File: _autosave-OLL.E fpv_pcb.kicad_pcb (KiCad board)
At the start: 6 copper layers, 47.6 x 41.5 mm, 141 parts, among them J1 Micro_SD_Card, J10 Conn_01x05_Pin, J2 RC, J8 reciver, J9 TYPE-C-31-M-12, M1 M1 front left, M2 M2 front right, M3 M3 rear right, M4 m4 rear left, Q1 2N7002, Q2 SUD45P03-09, SW1 SW_SPST, SW2 SW_SPST, U1 MP2315GJ, U10 AON7410, U11 UCC27511ADBV, U12 AON7410, U13 BMP280, U14 STM32H753VITx, U15 USBLC6-2SC6, U3 MP2315GJ, U4 ICM-42688-P, U5 UCC27511ADBV, U6 ul_AON7410, U7 UCC27511ADBV, U8 AON7410, U9 UCC27511ADBV, Y2 8HMz

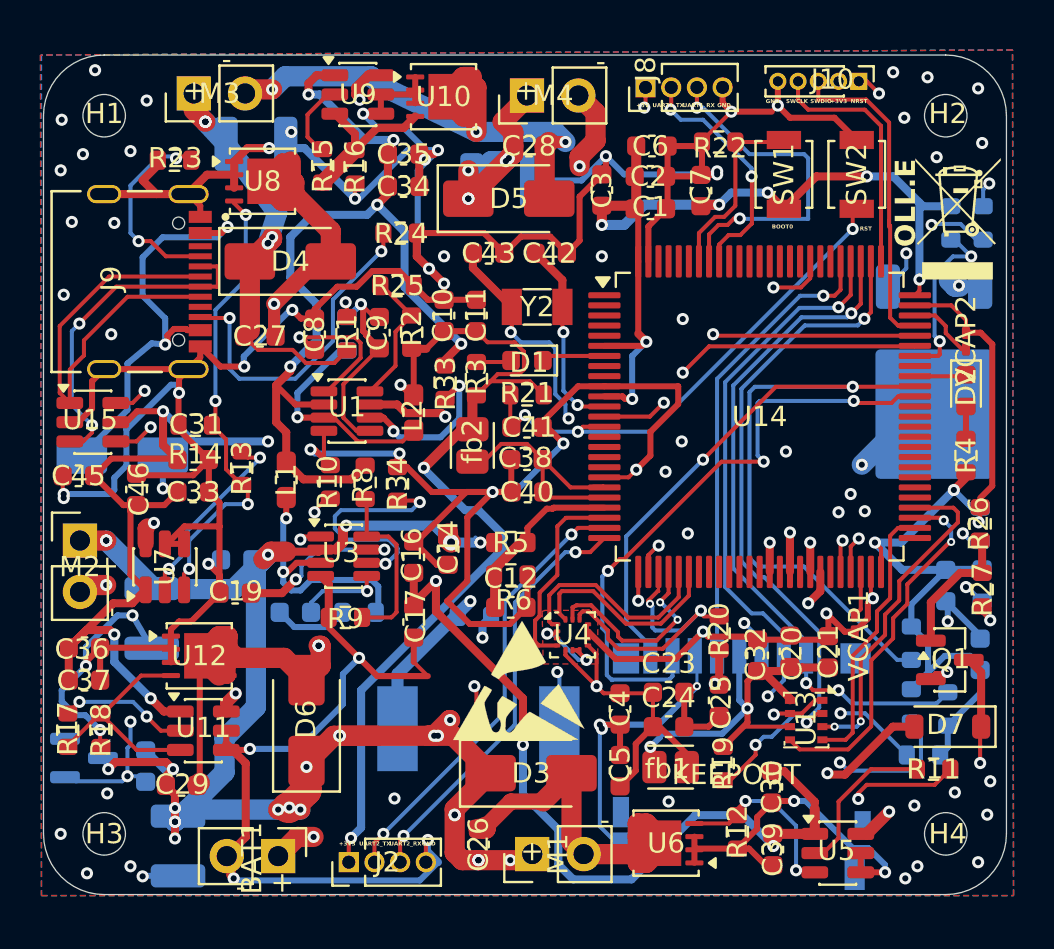
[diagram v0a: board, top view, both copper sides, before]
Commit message: update
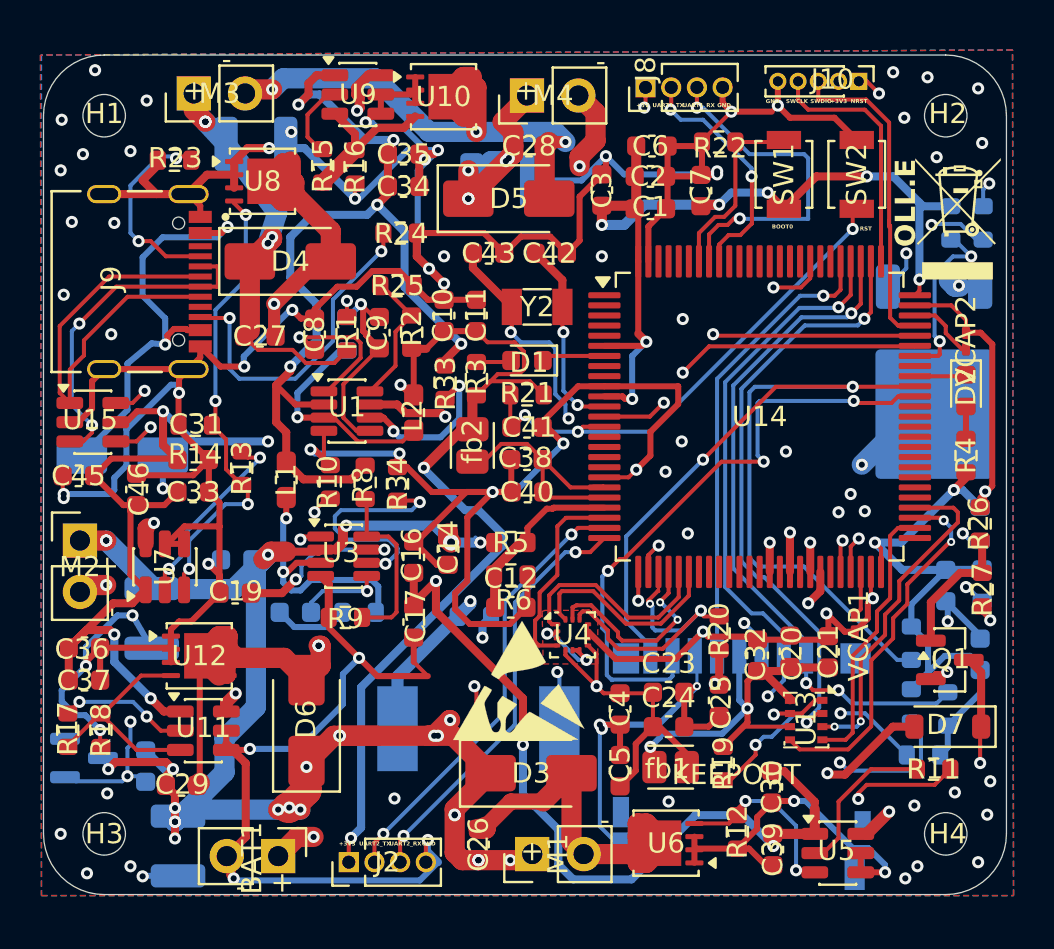
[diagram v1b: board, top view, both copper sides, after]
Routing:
- net +5V_FC: track 179.2 -> 182.3 mm
- net GND: track 410.3 -> 411.4 mm
- net MOTOR3: track 42.1 -> 43.2 mm
